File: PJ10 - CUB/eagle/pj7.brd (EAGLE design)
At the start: 49.5 x 49.5 mm, 69 parts, among them U2 PRTR5V0U2X, U3 CP210X_USB_UART, U4 STM32F103C8T, U5 HEX_CONVERTER, U6 74HC14D

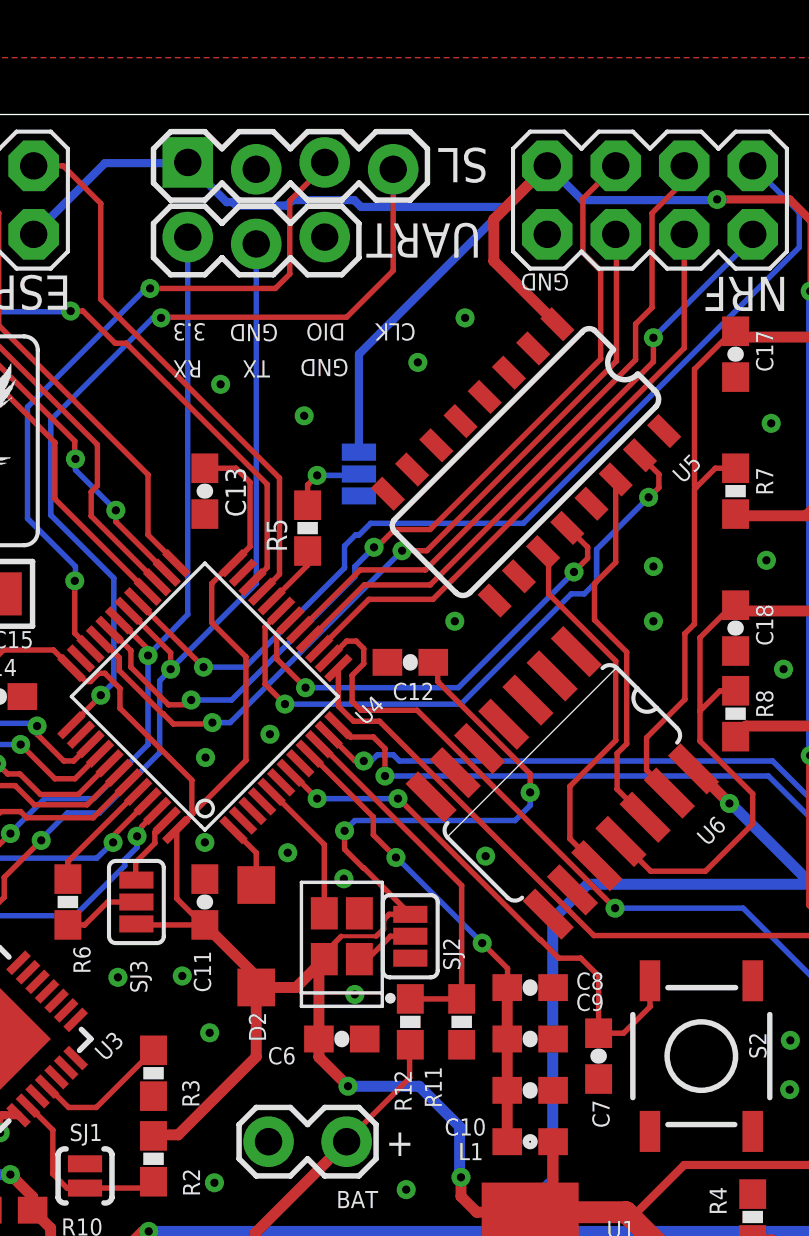
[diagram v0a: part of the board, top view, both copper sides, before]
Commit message: bak Nov 5
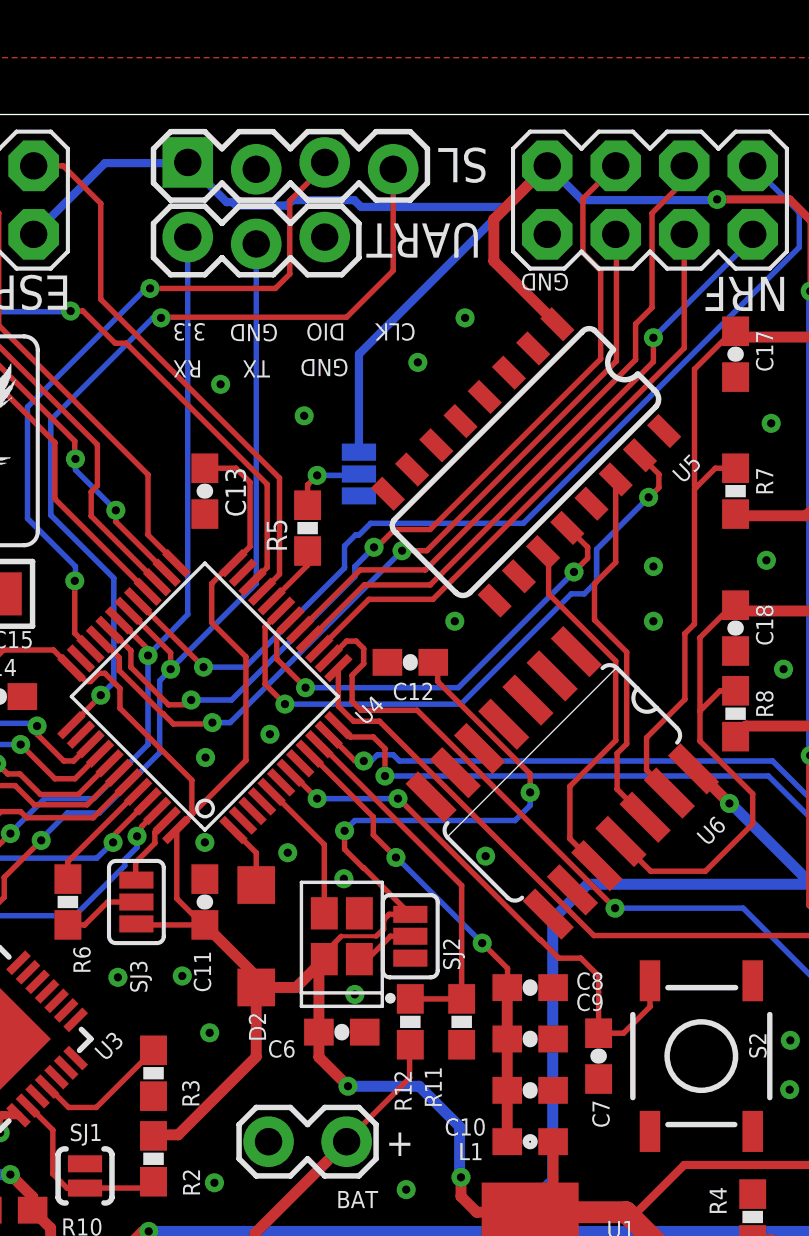
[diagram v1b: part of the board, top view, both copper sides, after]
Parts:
- moved C6 0.25 mm to (26.7, 15.5)
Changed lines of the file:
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@@
 <attribute name="NAME" x="10.3124" y="11.7602" size="0.635" layer="25" font="vector" rot="R270"/>
 </element>
-<element name="C6" library="SparkFun-Capacitors" package="0603-CAP" value="1.0uF" x="26.67" y="15.24" smashed="yes" rot="R180">
-<attribute name="PROD_ID" value="CAP-00868" x="26.67" y="15.24" size="1.778" layer="27" rot="R180" display="off"/>
-<attribute name="NAME" x="24.9682" y="14.9352" size="0.635" layer="25" font="vector" rot="R180"/>
+<element name="C6" library="SparkFun-Capacitors" package="0603-CAP" value="1.0uF" x="26.67" y="15.494" smashed="yes" rot="R180">
+<attribute name="PROD_ID" value="CAP-00868" x="26.67" y="15.494" size="1.778" layer="27" rot="R180" display="off"/>
+<attribute name="NAME" x="24.9682" y="15.1892" size="0.635" layer="25" font="vector" rot="R180"/>
 </element>
 <element name="C7" library="SparkFun-Capacitors" package="0603-CAP" value="1.0uF" x="36.195" y="14.605" smashed="yes" rot="R90">
@@
 <wire x1="34.505" y1="11.43" x2="34.505" y2="9.664" width="0.4064" layer="1"/>
 <wire x1="34.505" y1="9.664" x2="33.655" y2="8.814" width="0.4064" layer="1"/>
-<wire x1="25.82" y1="15.24" x2="25.82" y2="14.566" width="0.4064" layer="1"/>
+<wire x1="25.82" y1="15.494" x2="25.82" y2="14.566" width="0.4064" layer="1"/>
 <wire x1="25.82" y1="14.566" x2="26.8986" y2="13.4874" width="0.4064" layer="1"/>
 <via x="26.8986" y="13.4874" extent="1-16" drill="0.3048"/>
@@
 <wire x1="31.6738" y1="8.8138" x2="33.6548" y2="8.8138" width="0.4064" layer="1"/>
 <wire x1="33.6548" y1="8.8138" x2="33.655" y2="8.814" width="0.4064" layer="1"/>
-<wire x1="25.82" y1="15.24" x2="25.82" y2="18" width="0.4064" layer="1"/>
+<wire x1="25.82" y1="15.494" x2="25.82" y2="18" width="0.4064" layer="1"/>
 <wire x1="25.82" y1="18" x2="26.02" y2="18.2" width="0.4064" layer="1"/>
 <wire x1="23.495" y1="17.15" x2="24.97" y2="17.15" width="0.4064" layer="1"/>
@@
 <wire x1="20.955" y1="47.752" x2="20.955" y2="47.7266" width="0.3048" layer="16"/>
 <wire x1="20.955" y1="47.7266" x2="22.4028" y2="46.2788" width="0.3048" layer="16"/>
-<wire x1="32.9438" y1="46.2788" x2="33.782" y2="47.117" width="0.3048" layer="16"/>
-<wire x1="33.782" y1="47.117" x2="34.2646" y2="47.5996" width="0.3048" layer="16"/>
-<wire x1="34.2646" y1="47.5996" x2="34.29" y2="47.625" width="0.3048" layer="16"/>
+<wire x1="32.766" y1="46.101" x2="34.2646" y2="47.5996" width="0.3048" layer="16"/>
 <wire x1="20.955" y1="47.7266" x2="17.8816" y2="47.7266" width="0.3048" layer="16"/>
 <wire x1="17.8816" y1="47.7266" x2="15.24" y2="45.085" width="0.3048" layer="16"/>
@@
 <wire x1="27.1272" y1="46.355" x2="27.3812" y2="46.101" width="0.3048" layer="16"/>
 <wire x1="27.3812" y1="46.101" x2="32.766" y2="46.101" width="0.3048" layer="16"/>
-<wire x1="32.766" y1="46.101" x2="32.9438" y2="46.2788" width="0.3048" layer="16"/>
 </signal>
 <signal name="N$15">
